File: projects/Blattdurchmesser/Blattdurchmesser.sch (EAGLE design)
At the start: 17 parts, among them K1 TX2_RELAY", Q1 ARDUINOR3-NOIOREF-NOTEXT

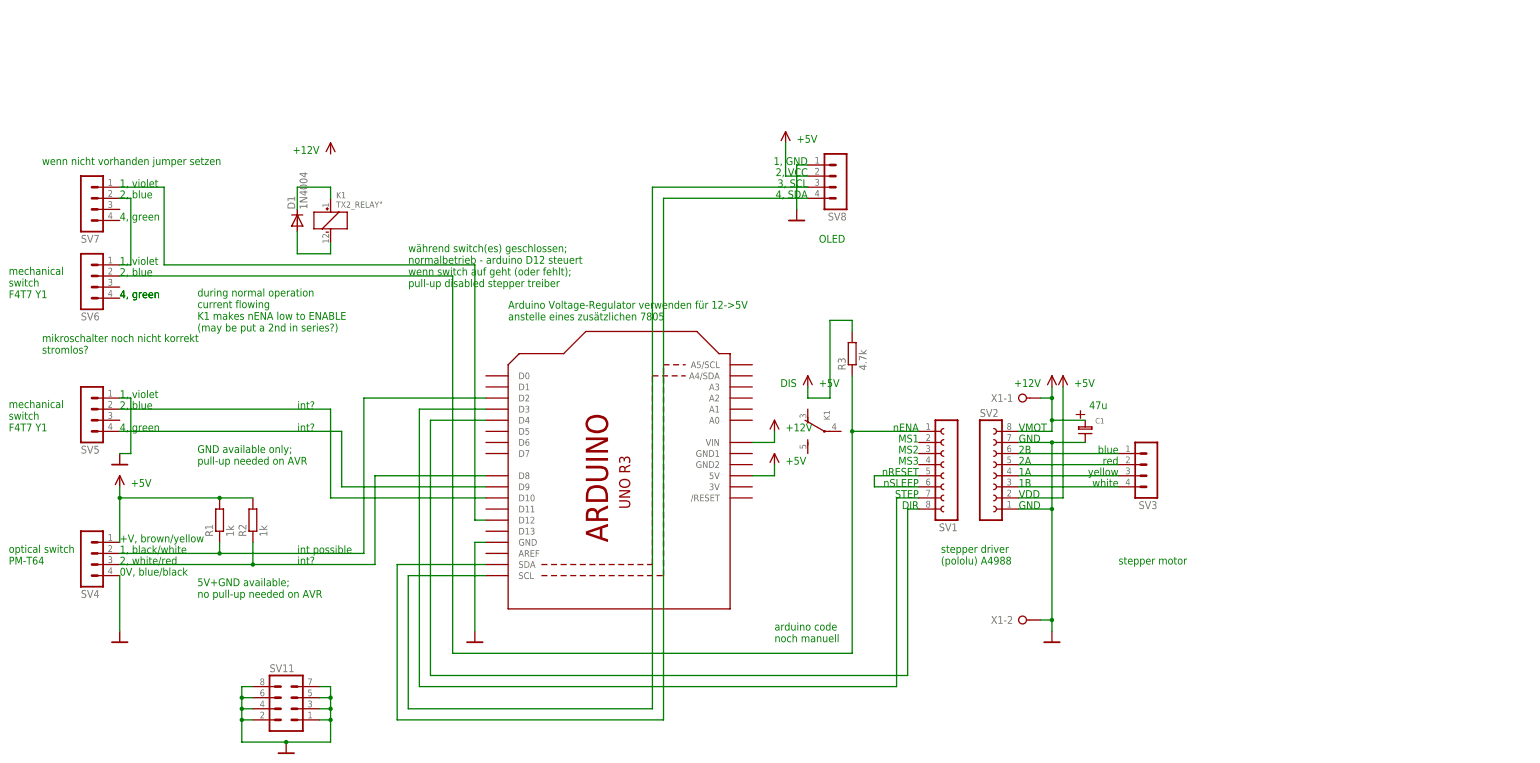
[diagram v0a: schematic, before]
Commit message: improvement; * rearranged schematic              * rearranged pcb
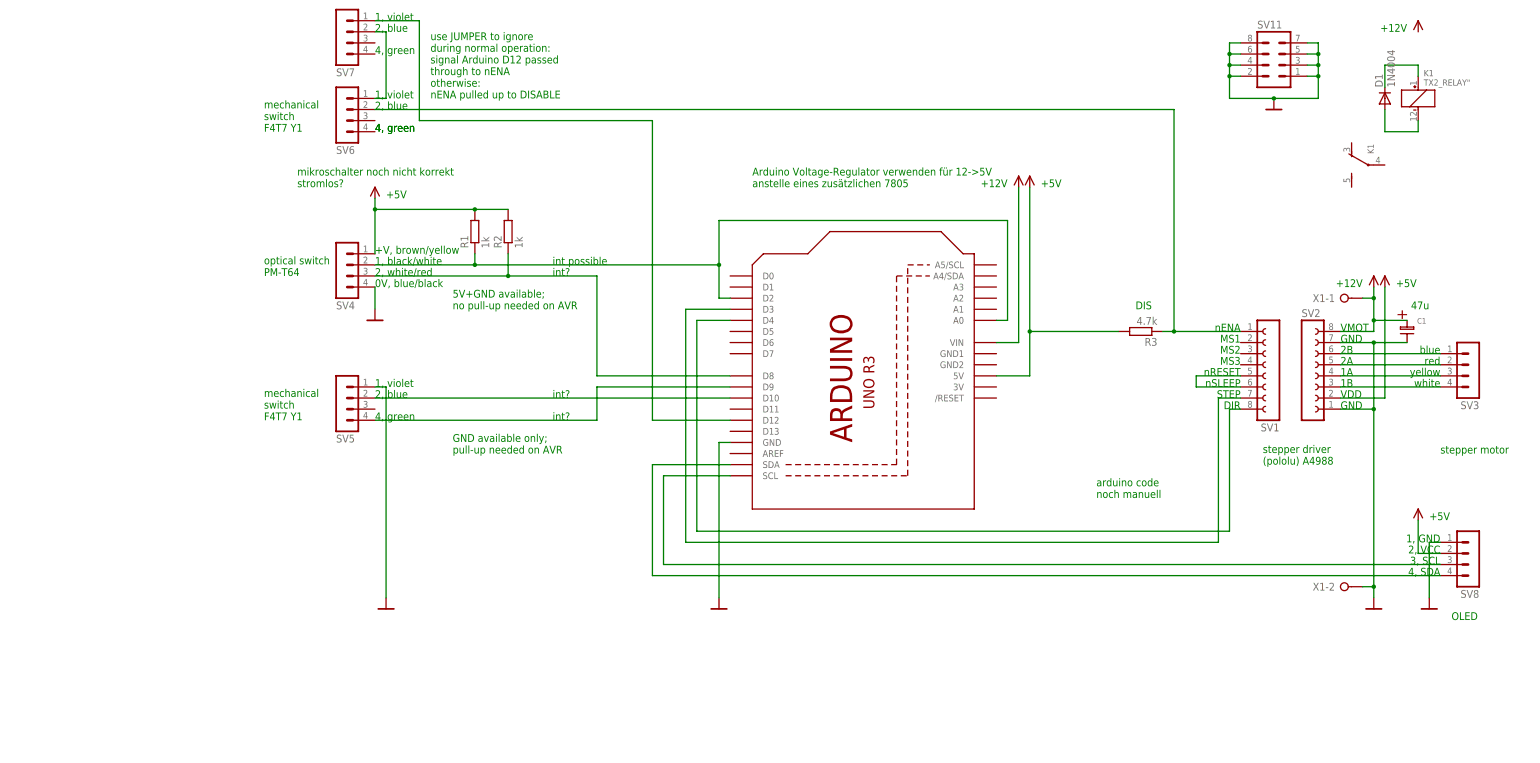
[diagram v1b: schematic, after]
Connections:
- net N$15: now also Q1.A0
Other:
- note added: "use JUMPER to ignore during normal operation: signal Arduino D12 passed through to nENA otherwise: nENA pulled up to DISABLE"
- note removed: "during normal operation current flowing K1 makes nENA low to ENABLE (may be put a 2nd in series?)"
- note removed: "wenn nicht vorhanden jumper setzen"
- note removed: "während switch(es) geschlossen; normalbetrieb - arduino D12 steuert wenn switch auf geht (oder fehlt); pull-up disabled stepper treiber"
- moved on the sheet: C1, D1, K1, R1, R2, R3, SV1, SV11, SV2, SV3, SV4, SV5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
